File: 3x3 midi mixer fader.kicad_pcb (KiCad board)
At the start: 2 copper layers, 159 x 75.3 mm, 76 parts, among them J1 B1, J2 B2, J3 B3, J4 B4, Q0 BSS138, U0 ADS1115IDGS, U1 W25Q128JVS

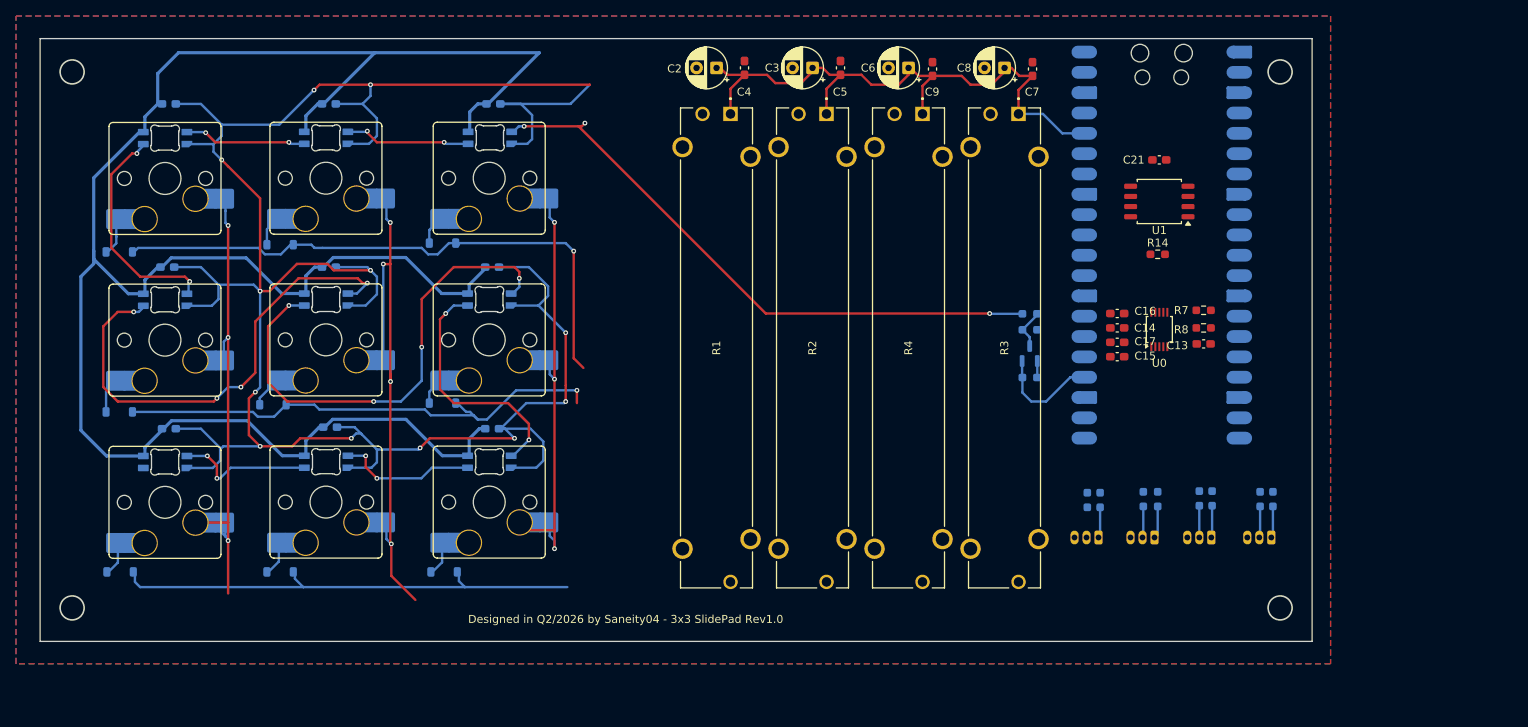
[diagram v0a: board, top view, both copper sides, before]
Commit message: Add files via upload
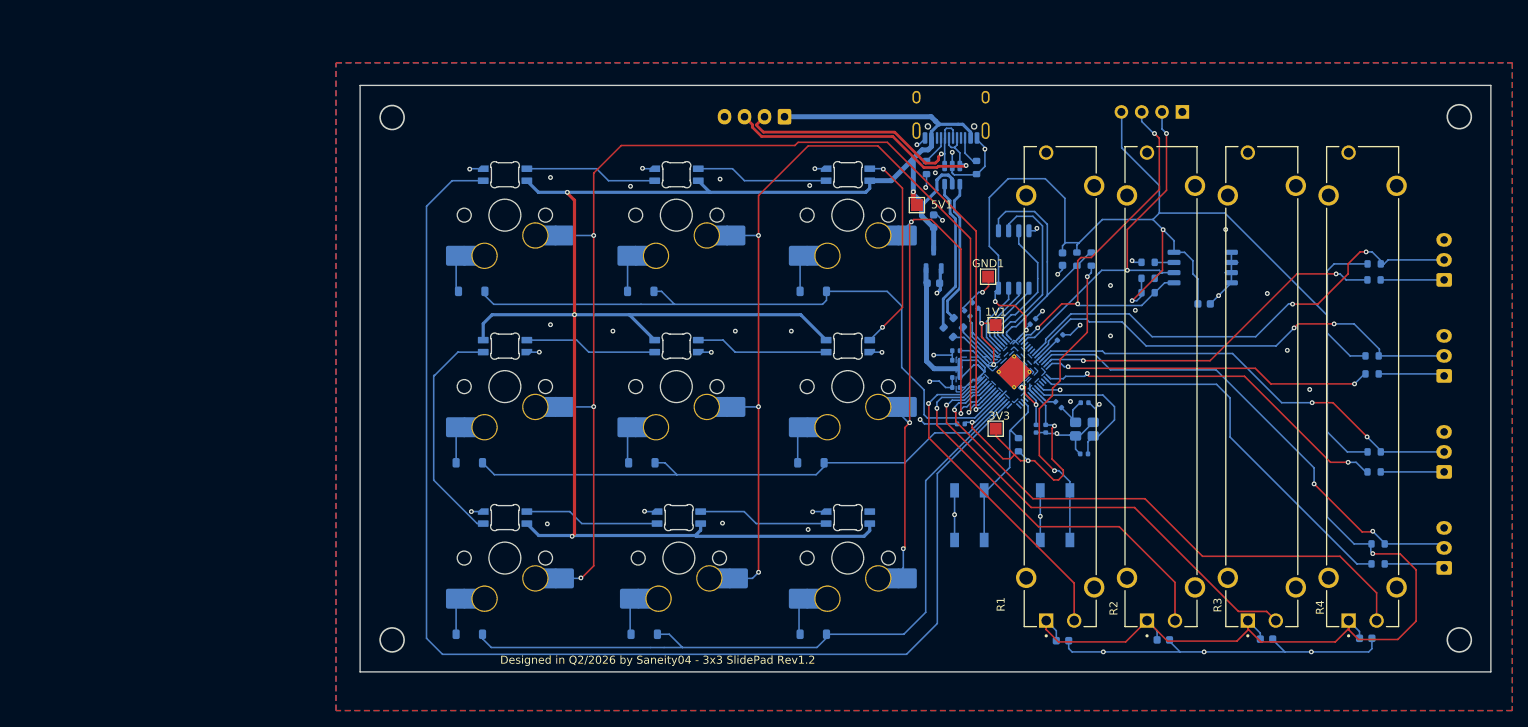
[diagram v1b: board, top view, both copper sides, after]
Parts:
- removed A0: RaspberryPi_Pico, Module:RaspberryPi_Pico_Common_SMD
- removed C14, C16, C17, C19, C20: 0.1uF, Capacitor_SMD:C_0603_1608Metric_Pad1.08x0.95mm_HandSolder
- removed D0: 1N4148W, Diode_SMD:D_SOD-123
- removed Q0: BSS138, Package_TO_SOT_SMD:SOT-23
- removed R5: 10k, Resistor_SMD:R_0603_1608Metric_Pad0.98x0.95mm_HandSolder
- removed R8: 4.7k, Resistor_SMD:R_0603_1608Metric_Pad0.98x0.95mm_HandSolder
- removed RGB0: WS2812B, PCM_marbastlib-mx:LED_MX_6028R-ROT
- removed S0: PG151101S11, PCM_marbastlib-mx:SW_MX_HS_CPG151101S11_1u
- removed U0: ADS1115IDGS, Package_SO:TSSOP-10_3x3mm_P0.5mm
- added 1V1: 1.1V, TestPoint:TestPoint_Pad_1.5x1.5mm, F.Cu at (162.9, 88.7)
- added 3V3: 3.3V, TestPoint:TestPoint_Pad_1.5x1.5mm, F.Cu at (162.9, 101.6)
- added 5V1: 5V, TestPoint:TestPoint_Pad_1.5x1.5mm, F.Cu at (153.1, 73.7)
- added C1: 100n, Capacitor_SMD:C_0603_1608Metric, B.Cu at (171.3, 128.1)
- added C25: 100n, Capacitor_SMD:C_0402_1005Metric, B.Cu at (168.0, 101.6)
- added C26: 15p, Capacitor_SMD:C_0402_1005Metric, B.Cu at (174.0, 104.8)
- added D9: 1N4148W, Diode_SMD:D_SOD-123, B.Cu at (97.1, 127.3)
- added GND1: GND, TestPoint:TestPoint_Pad_1.5x1.5mm, F.Cu at (162.0, 82.6)
- added J5: B4, Connector_JST:JST_XH_B3B-XH-A_1x03_P2.50mm_Vertical, B.Cu at (219.0, 119.0)
- added J6: Conn_01x04, Connector_JST:JST_XH_B4B-XH-A_1x04_P2.50mm_Vertical, B.Cu at (136.6, 62.6)
- added J7: Conn_01x04, Connector_PinHeader_2.54mm:PinHeader_1x04_P2.54mm_Vertical, B.Cu at (186.3, 62.0)
- added R19: 10k, Resistor_SMD:R_0603_1608Metric, B.Cu at (210.3, 104.5)
- added R20: 220, Resistor_SMD:R_0603_1608Metric, B.Cu at (210.0, 94.8)
- added R21: 1k, Resistor_SMD:R_0402_1005Metric, B.Cu at (170.8, 98.6)
- added R22: 10k, Resistor_SMD:R_0603_1608Metric, B.Cu at (210.0, 92.5)
- added R23: 10k, Resistor_SMD:R_0603_1608Metric, B.Cu at (165.8, 103.6)
- added R24: 220, Resistor_SMD:R_0603_1608Metric, B.Cu at (210.8, 118.5)
- added R25: 10k, Resistor_SMD:R_0603_1608Metric, B.Cu at (210.8, 116.0)
- added RGB9: WS2812B, PCM_marbastlib-mx:LED_MX_6028R, B.Cu at (144.5, 112.7)
- added S9: PG151101S11, PCM_marbastlib-mx:SW_MX_HS_CPG151101S11_1u, B.Cu at (101.6, 117.8)
- added SW1: SW_SPST, Button_Switch_SMD:SW_SPST_SKQG_WithStem, B.Cu at (170.4, 112.4)
- added SW2: SW_SPST, Button_Switch_SMD:SW_SPST_SKQG_WithStem, B.Cu at (159.7, 112.4)
- added U2: W25Q16JVSS, Package_SO:SOIC-8_5.3x5.3mm_P1.27mm, B.Cu at (165.2, 80.5)
- added U3: 24LC256, Package_SO:SOIC-8_5.3x5.3mm_P1.27mm, B.Cu at (188.8, 81.5)
- added U4: XC6206PxxxMR, Package_TO_SOT_SMD:SOT-23-3, B.Cu at (155.2, 80.4)
- added U6: RP2040, Package_DFN_QFN:QFN-56-1EP_7x7mm_P0.4mm_EP3.2x3.2mm_ThermalVias, B.Cu at (165.3, 94.5)
- added Y1: Crystal_GND24, Crystal:Crystal_SMD_3225-4Pin_3.2x2.5mm, B.Cu at (174.0, 101.7)
- C10, C11, C12, C18, C22, C24: value 0.1uF -> 100n; footprint Capacitor_SMD:C_0603_1608Metric_Pad1.08x0.95mm_HandSolder -> Capacitor_SMD:C_0402_1005Metric
- C13, C15: value 0.1uF -> 1u; footprint Capacitor_SMD:C_0603_1608Metric_Pad1.08x0.95mm_HandSolder -> Capacitor_SMD:C_0402_1005Metric; moved to B.Cu
- C2, C3, C6, C8: value 10uF -> 100n; footprint Capacitor_THT:CP_Radial_D5.0mm_P2.50mm -> Capacitor_SMD:C_0603_1608Metric; moved to B.Cu
- C21, C9: value 0.1uF -> 100n; footprint Capacitor_SMD:C_0603_1608Metric_Pad1.08x0.95mm_HandSolder -> Capacitor_SMD:C_0402_1005Metric; moved to B.Cu
- C23: value 0.1uF -> 15p; footprint Capacitor_SMD:C_0603_1608Metric_Pad1.08x0.95mm_HandSolder -> Capacitor_SMD:C_0402_1005Metric
- C4: value 0.1uF -> 100n; footprint Capacitor_SMD:C_0603_1608Metric_Pad1.08x0.95mm_HandSolder -> Capacitor_SMD:C_0603_1608Metric; moved to B.Cu
- C5, C7: value 0.1uF -> 10u; footprint Capacitor_SMD:C_0603_1608Metric_Pad1.08x0.95mm_HandSolder -> Capacitor_SMD:C_0603_1608Metric; moved to B.Cu
- J1: value B1 -> USB_C_Receptacle_USB2.0_16P; footprint Connector_JST:JST_ZH_B3B-ZR_1x03_P1.50mm_Vertical -> Connector_USB:USB_C_Receptacle_HRO_TYPE-C-31-M-12
- J2: value B2 -> B1; footprint Connector_JST:JST_ZH_B3B-ZR_1x03_P1.50mm_Vertical -> Connector_JST:JST_XH_B3B-XH-A_1x03_P2.50mm_Vertical
- J3: footprint Connector_JST:JST_ZH_B3B-ZR_1x03_P1.50mm_Vertical -> Connector_JST:JST_XH_B3B-XH-A_1x03_P2.50mm_Vertical
- J4: value B4 -> B2; footprint Connector_JST:JST_ZH_B3B-ZR_1x03_P1.50mm_Vertical -> Connector_JST:JST_XH_B3B-XH-A_1x03_P2.50mm_Vertical
- R10: value 10k -> 1K; footprint Resistor_SMD:R_0603_1608Metric_Pad0.98x0.95mm_HandSolder -> Resistor_SMD:R_0603_1608Metric
- R11: value 220 -> DNF; footprint Resistor_SMD:R_0603_1608Metric_Pad0.98x0.95mm_HandSolder -> Resistor_SMD:R_0603_1608Metric
- R12: value 10k -> 220; footprint Resistor_SMD:R_0603_1608Metric_Pad0.98x0.95mm_HandSolder -> Resistor_SMD:R_0603_1608Metric
- R13, R16, R9: footprint Resistor_SMD:R_0603_1608Metric_Pad0.98x0.95mm_HandSolder -> Resistor_SMD:R_0603_1608Metric
- R14: value 10k -> 3.3k; footprint Resistor_SMD:R_0603_1608Metric_Pad0.98x0.95mm_HandSolder -> Resistor_SMD:R_0603_1608Metric; moved to B.Cu
- R15, R18: value 220 -> 27; footprint Resistor_SMD:R_0603_1608Metric_Pad0.98x0.95mm_HandSolder -> Resistor_SMD:R_0603_1608Metric
- R17: value 220 -> 3.3k; footprint Resistor_SMD:R_0603_1608Metric_Pad0.98x0.95mm_HandSolder -> Resistor_SMD:R_0603_1608Metric
- R6: value 10k -> 5.1K; footprint Resistor_SMD:R_0603_1608Metric_Pad0.98x0.95mm_HandSolder -> Resistor_SMD:R_0603_1608Metric
- R7: value 4.7k -> 5.1K; footprint Resistor_SMD:R_0603_1608Metric_Pad0.98x0.95mm_HandSolder -> Resistor_SMD:R_0603_1608Metric; moved to B.Cu
- RGB1, RGB2, RGB3, RGB7, RGB8: footprint PCM_marbastlib-mx:LED_MX_6028R-ROT -> PCM_marbastlib-mx:LED_MX_6028R
- U1: value W25Q128JVS -> USBLC6-2SC6; footprint Package_SO:SOIC-8_5.3x5.3mm_P1.27mm -> Package_TO_SOT_SMD:SOT-23-6; moved to B.Cu
- moved C12 115.2 mm to (171.0, 90.2), turned to 45 degrees
- moved C4 105.4 mm to (209.2, 127.8), turned to 0 degrees
- moved C24 99.0 mm to (158.6, 101.0), turned to 180 degrees
- moved C23 94.4 mm to (174.1, 98.3)
- moved S7 92.6 mm to (144.5, 74.9)
- moved C3 91.2 mm to (196.8, 127.9), turned to 0 degrees
- moved C2 90.7 mm to (183.9, 128.0), turned to 0 degrees
- moved RGB6 85.5 mm to (144.5, 91.3)
- moved C11 84.0 mm to (159.4, 87.2), turned to 135 degrees
- moved D7 75.3 mm to (140.1, 84.4)
- moved D4 73.4 mm to (140.1, 127.3)
- moved D1 71.7 mm to (139.9, 105.9)
- moved D5 71.3 mm to (119.0, 127.3)
- moved S1 70.2 mm to (144.5, 96.3)
- moved C22 69.2 mm to (169.2, 101.6), turned to -90 degrees
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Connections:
- C10 pad 1: +5V -> +1V1
- C11 pad 1: +5V -> +3.3V
- C12 pad 1: +5V -> +3.3V
- C13 pad 1: +3.3V -> +1V1
- C15 pad 1: Fader 1 -> +3.3V
- C18 pad 1: +5V -> +3.3V
- C22 pad 1: +5V -> +3.3V
- C23 pad 1: +5V -> Net-(C23-Pad1)
- C24 pad 1: +5V -> +3.3V
- C5 pad 1: +3.3V -> +5V
- D1 pad 1: Row 1 -> /Row_2
- D2 pad 1: Row 1 -> /Row_1
- D3 pad 1: Row 2 -> /Row_1
- D4 pad 1: Row 2 -> /Row_3
- D5 pad 1: Row 2 -> /Row_3
- D6 pad 1: Row 3 -> /Row_2
- D7 pad 1: Row 3 -> /Row_1
- D8 pad 1: Row 3 -> /Row_2
- J2 pad 2: B2 -> /Button_1
- J3 pad 2: B3 -> /Button_3
- J4 pad 2: B4 -> /Button_2
- R1 pad 2: Fader 4 -> /Fader_4
- R10 pad 1: +3.3V -> Net-(SW1-B)
- R10 pad 2: WS2812IN_LV -> /~{QSPI_SS}
- R11 pad 1: Net-(RGB1-DIN) -> +3.3V
- R11 pad 2: WS2812IN_HV -> /~{QSPI_SS}
- R12 pad 1: +3.3V -> Net-(J2-Pin_1)
- R12 pad 2: B3 -> /LED_1
- R13 pad 1: +3.3V -> /Button_1
- R13 pad 2: B4 -> +3.3V
- R14 pad 2: SPI_CS -> /EEPROM_SDA
- R15 pad 1: Net-(J1-Pin_1) -> /USB_D+
- R15 pad 2: LED1 -> Net-(U6-USB_DP)
- R16 pad 2: LED2 -> /LED_3
- R17 pad 1: Net-(J2-Pin_1) -> +3.3V
- R17 pad 2: LED3 -> /EEPROM_SCL
- R18 pad 1: Net-(J4-Pin_1) -> Net-(U6-USB_DM)
- R18 pad 2: LED4 -> /USB_D-
- R2 pad 2: Fader 3 -> /Fader_3
- R3 pad 2: Fader 1 -> /Fader_2
- R4 pad 2: Fader 2 -> /Fader_1
- R6 pad 1: +3.3V -> Net-(J1-CC2)
- R6 pad 2: B2 -> GND
- R7 pad 1: +3.3V -> Net-(J1-CC1)
- R7 pad 2: SCL -> GND
- R9 pad 1: +5V -> Net-(U3-WP)
- R9 pad 2: WS2812IN_HV -> GND
- RGB1 pad 3: Net-(RGB1-DIN) -> /WS2812_RGB
- RGB2 pad 3: Net-(RGB0-DOUT) -> Net-(RGB1-DOUT)
- RGB3 pad 3: Net-(RGB1-DOUT) -> Net-(RGB2-DOUT)
- RGB4 pad 3: Net-(RGB2-DOUT) -> Net-(RGB4-DIN)
- RGB5 pad 2: Net-(RGB5-DOUT) -> Net-(RGB4-DIN)
- RGB5 pad 3: Net-(RGB3-DOUT) -> Net-(RGB5-DIN)
- RGB6 pad 2: Net-(RGB0-DIN) -> Net-(RGB5-DIN)
- RGB6 pad 3: Net-(RGB5-DOUT) -> Net-(RGB3-DOUT)
- RGB8 pad 2: unconnected-(RGB8-DOUT-Pad2) -> Net-(RGB8-DOUT)
- S1 pad 1: Column 2 -> /Col_3
- S2 pad 1: Column 3 -> /Col_2
- S3 pad 1: Column 1 -> /Col_1
- S4 pad 1: Column 1 -> /Col_3
- S4 pad 2: Net-(D6-A) -> Net-(D4-A)
- S5 pad 1: Column 2 -> /Col_2
- S5 pad 2: Net-(D7-A) -> Net-(D5-A)
- S6 pad 1: Column 2 -> /Col_1
- S6 pad 2: Net-(D4-A) -> Net-(D6-A)
- S7 pad 1: Column 3 -> /Col_3
- S7 pad 2: Net-(D8-A) -> Net-(D7-A)
- S8 pad 1: Column 3 -> /Col_2
- S8 pad 2: Net-(D5-A) -> Net-(D8-A)
- U1 pad 1: SPI_CS -> /USB_CON_D-
- U1 pad 2: SPI_MISO -> GND
- U1 pad 3: +3.3V -> /USB_CON_D+
- U1 pad 4: GND -> /USB_D+
- U1 pad 5: SPI_MOSI -> +5V
- U1 pad 6: SPI_CLK -> /USB_D-
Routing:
- net +3.3V: track 79.3 -> 353.7 mm, vias 0 -> 8
- net /WS2812_RGB: track 0.00 -> 159.8 mm
- net GND: track 293.6 -> 144.5 mm, vias 12 -> 53
- net /Col_1: track 0.00 -> 140.7 mm, vias 0 -> 4
- net /Col_2: track 0.00 -> 115.9 mm, vias 0 -> 4
- net /Row_3: track 0.00 -> 92.8 mm
- net /Row_1: track 0.00 -> 83.8 mm
- net /Col_3: track 0.00 -> 83.1 mm, vias 0 -> 4
- net Column 2: track 77.4 -> 0.00 mm, vias 4 -> 0
- net Net-(RGB1-DIN): track 74.6 -> 0.00 mm, vias 3 -> 0
- net /Row_2: track 0.00 -> 73.2 mm
- net Row 1: track 72.9 -> 0.00 mm, vias 1 -> 0
- net /Fader_1: track 0.00 -> 72.2 mm, vias 0 -> 1
- net Row 2: track 63.5 -> 0.00 mm, vias 1 -> 0
- net Column 3: track 63.2 -> 0.00 mm, vias 3 -> 0
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- added copper zone on B.Cu, net +1V1
- added copper zone on B.Cu, net +3.3V
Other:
- board size 159 x 75.3 mm -> 141.3 x 73.3 mm
- board text added: "BOOTSEL"
- board text added: "Designed in Q2/2026 by Saneity04 - 3x3 SlidePad Rev1.2"
- board text added: "RESET"
- board text removed: "+S-"
- board text removed: "Designed in Q2/2026 by Saneity04 - 3x3 SlidePad Rev1.0"
